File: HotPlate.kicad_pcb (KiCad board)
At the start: 2 copper layers, 88 x 161.4 mm, 38 parts, among them J2 ICSP, U1 LMT85LP

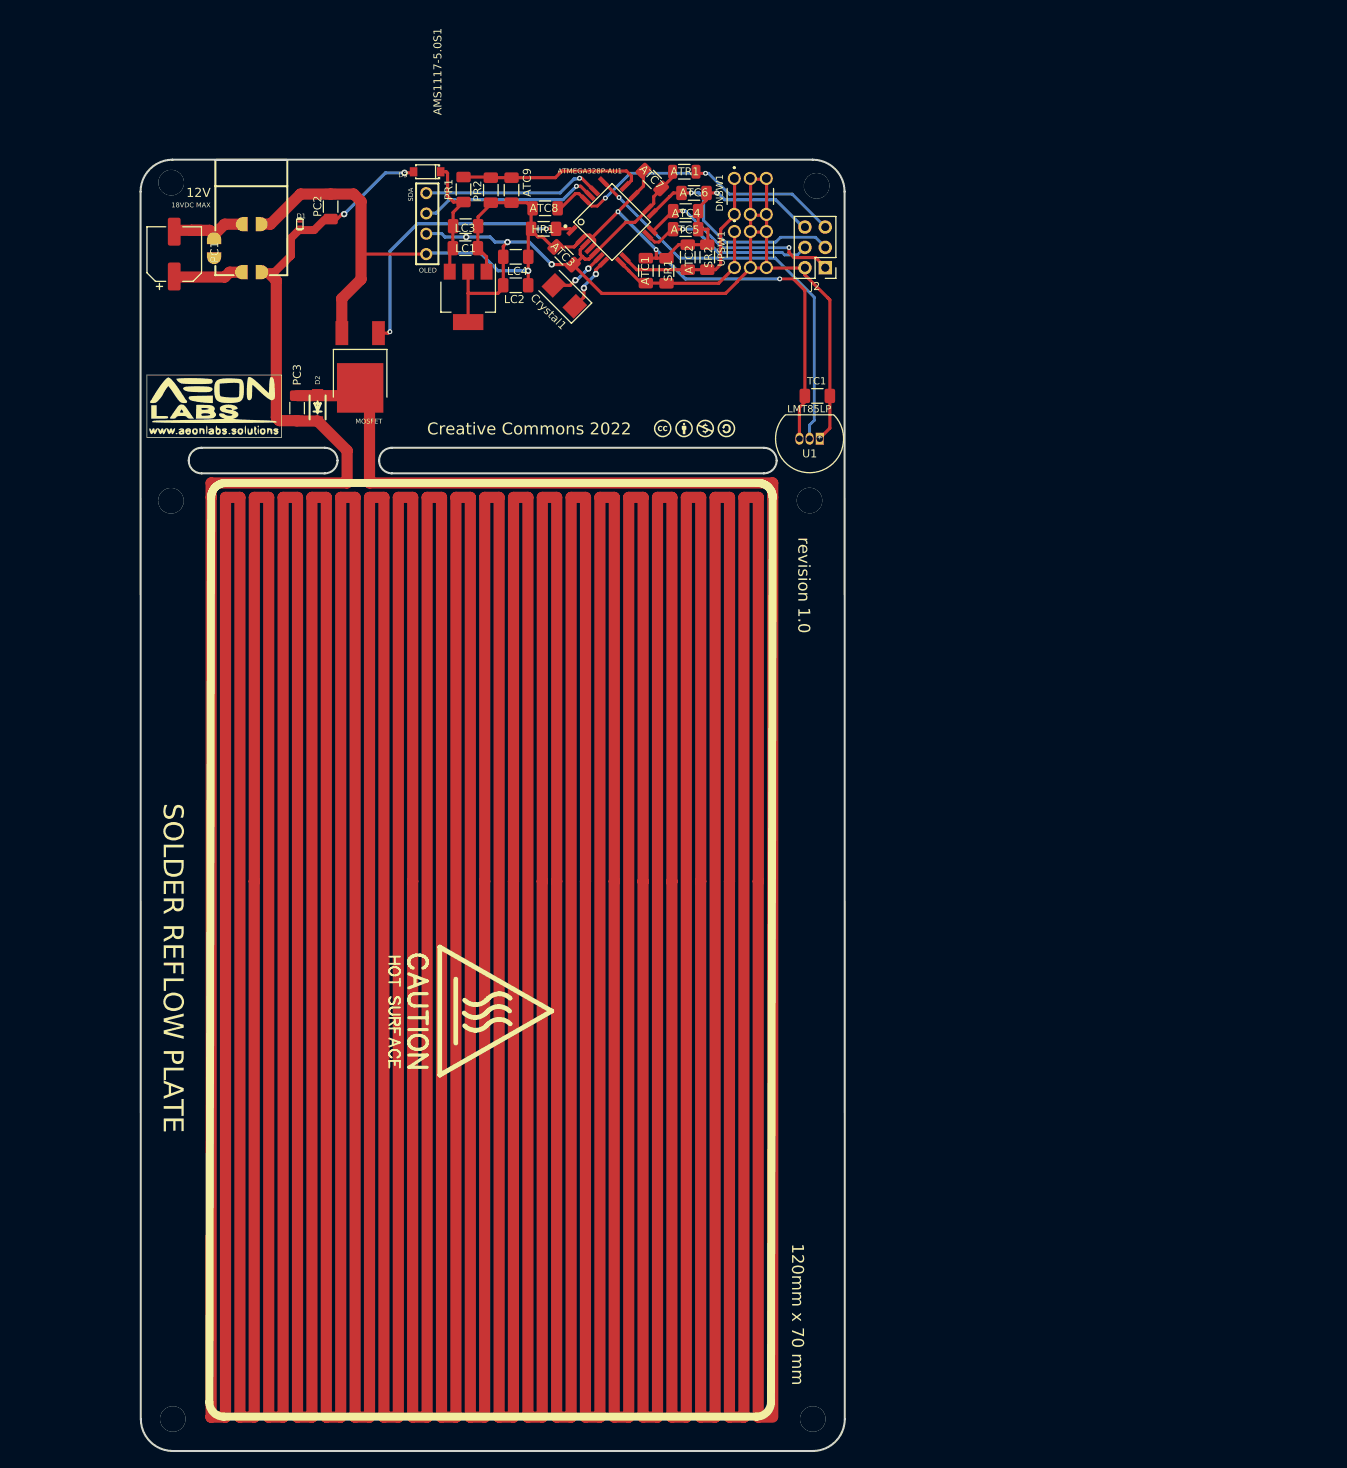
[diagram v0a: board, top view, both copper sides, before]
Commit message: update
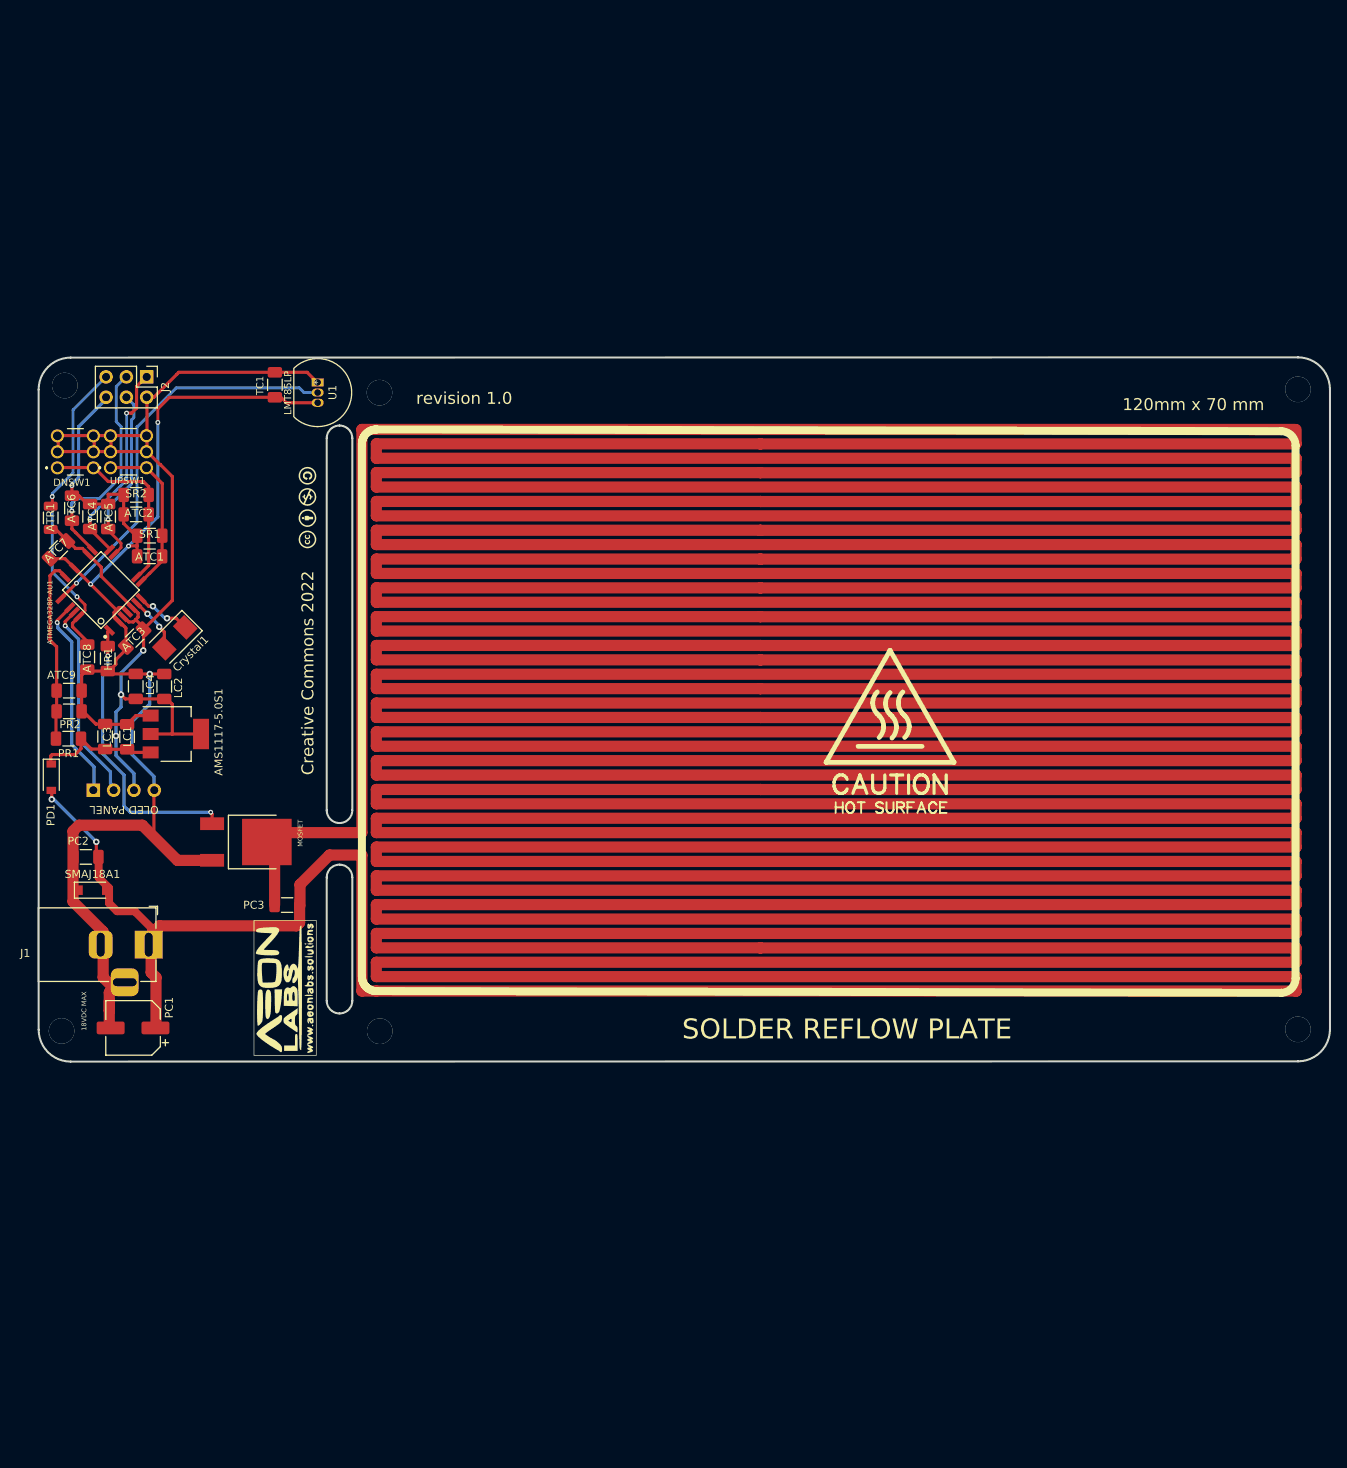
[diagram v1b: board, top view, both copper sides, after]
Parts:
- removed 12V: DC-005-5A-2.5, easyeda:DC-IN-TH_DC-005-5A-2.5
- removed D1: PESDMC2FD18VB, easyeda:SOD-882_L1.0-W0.6-BI
- removed D2: MM1Z24, easyeda:SOD-123_L2.8-W1.8-LS3.7-FD
- removed D3: DSR1M_C908221, easyeda:SOD-123_L2.8-W1.8-LS3.7-RD
- removed OLED: SDA, easyeda:OLED_0.91_128X32
- added 0.91"OLED1: Conn_01x04_Female, Display:SSD1306-0.91-OLED-4pin-128x32, B.Cu at (73.2, 63.9)
- added J1: Barrel_Jack_Switch, Connector_BarrelJack:BarrelJack_Horizontal, F.Cu at (82.3, 119.7)
- added PD1: D, Diode_SMD:D_SOD-123, F.Cu at (70.1, 98.7)
- added SMAJ18A1: SMAJ18A, Diode_SMD:D_SOD-123, F.Cu at (75.3, 112.8)
- moved PC1 96.9 mm to (80.3, 130.1), turned to 180 degrees
- moved DNSW1 92.0 mm to (70.9, 60.1), turned to 0 degrees
- moved ATR1 90.2 mm to (70.0, 66.3), turned to 90 degrees
- moved ATC7 87.5 mm to (71.0, 70.3), turned to -135 degrees
- moved ATC6 87.2 mm to (72.7, 65.1), turned to 90 degrees
- moved PC2 86.9 mm to (74.4, 108.7), turned to 180 degrees
- moved J2 85.9 mm to (82.0, 48.7), turned to -90 degrees
- moved PR1 84.6 mm to (72.3, 93.9), turned to 180 degrees
- moved PR2 83.8 mm to (72.3, 90.5), turned to 180 degrees
- moved ATC4 83.7 mm to (75.0, 66.1), turned to 90 degrees
- moved ATC9 83.5 mm to (72.3, 87.9), turned to 0 degrees
- moved UPSW1 83.4 mm to (77.5, 60.1), turned to 0 degrees
- moved ATC5 80.6 mm to (77.2, 66.2), turned to 90 degrees
- moved ATC8 80.1 mm to (74.6, 83.7), turned to 90 degrees
- moved ATMEGA328P-AU1 78.7 mm to (76.3, 75.3), turned to 135 degrees
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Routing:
- net Element: track 28.9 -> 4830.0 mm, vias 0 -> 2
- net VCC: track 4800.9 -> 0.00 mm, vias 1 -> 0
- net /GND: track 173.1 -> 197.8 mm
- net 0V: track 21.9 -> 0.00 mm
- net GATE: track 16.4 -> 0.00 mm, vias 1 -> 0
- net Gate: track 21.2 -> 37.6 mm, vias 1 -> 2
- net SDAOLED: track 22.5 -> 24.9 mm
- net SCKOLED: track 22.4 -> 24.8 mm
- net /5V0: track 140.6 -> 142.7 mm
- net (no net): vias 7 -> 6
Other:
- board size 88 x 161.4 mm -> 161.4 x 88 mm
- board text added: "OLED PANEL"
